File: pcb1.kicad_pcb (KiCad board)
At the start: 2 copper layers, 49.5 x 49.5 mm, 68 parts, among them P1 CONN_01X06, P10 M1, P11 M2, P12 CONN_01X02, P2 CONN_01X06, P3 CONN_01X06, P4 CONN_01X06, P5 UART, P6 SWD, Q1 IRF9540N, U1 74AHC1G14, U10 HL293D, U2 LTV-358T, U3 LTV-358T, U4 LM7812CT, U5 74AHC1G14, U6 STM32F030C6Tx, U7 LM7805CT, U8 LM1117-3.3, U9 HL293D

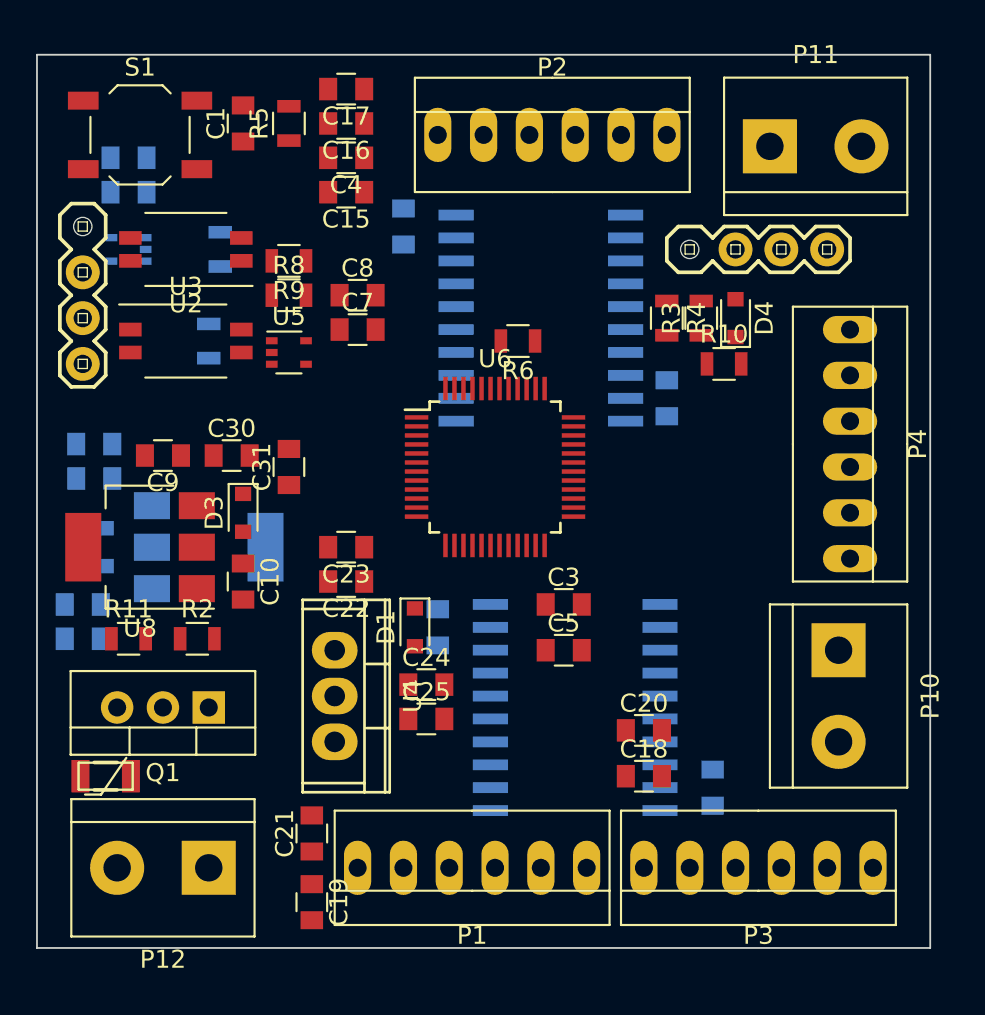
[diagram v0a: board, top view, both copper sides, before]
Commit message: 5x5
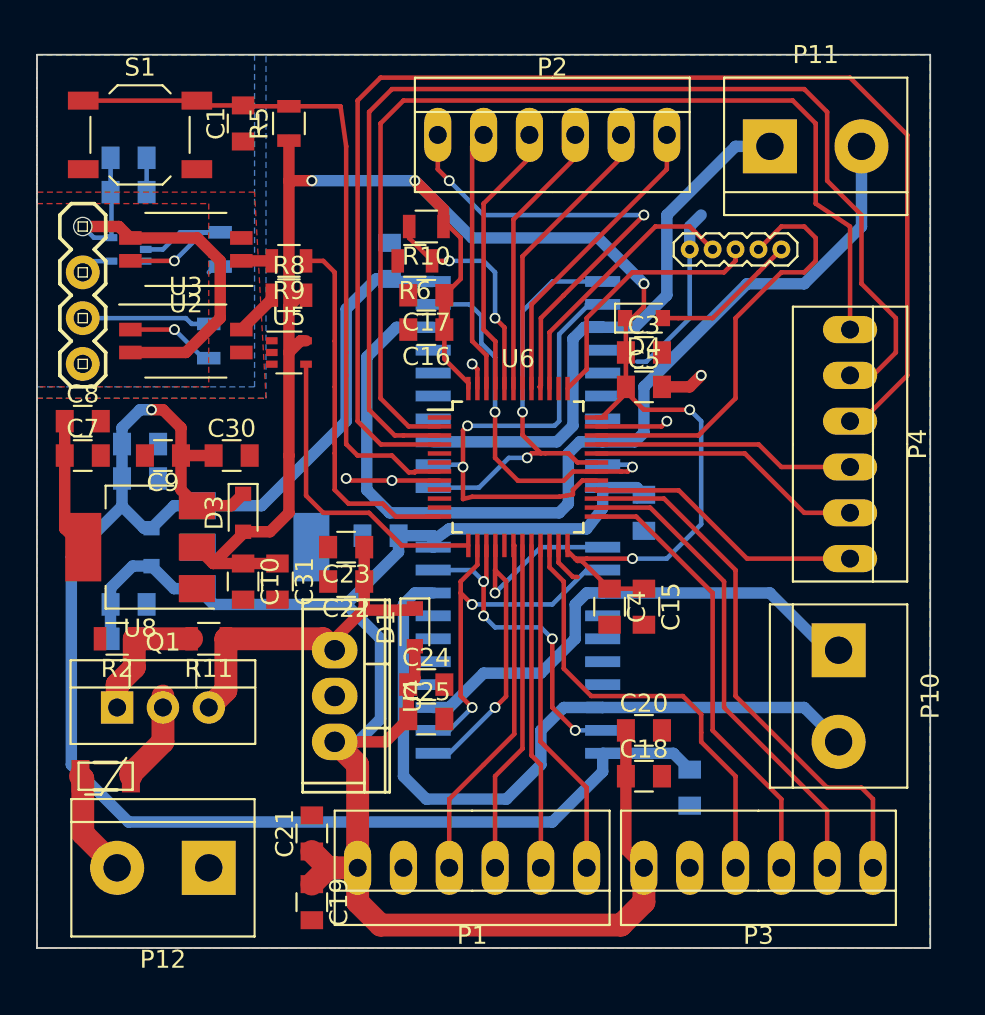
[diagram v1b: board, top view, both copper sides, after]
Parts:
- removed R3, R4: 100k, Resistors_SMD:R_0805
- P6: value SWD -> CONN_01X05; footprint SparkFun:SparkFun-1X04 -> SparkFun:SparkFun-1X05-1.27MM
- U6: value STM32F030C6Tx -> STM32F103C6Tx
- moved C4 28.9 mm to (219.7, 81.4), turned to 270 degrees
- moved C15 28.3 mm to (221.6, 81.4), turned to 270 degrees
- moved R10 18.2 mm to (209.6, 60.3), turned to 180 degrees
- moved C7 16.8 mm to (190.5, 73.0)
- moved C8 16.8 mm to (190.5, 71.1)
- moved C5 15.3 mm to (221.6, 69.2)
- moved C3 14.7 mm to (221.6, 67.3)
- moved C16 12.3 mm to (209.6, 66.0)
- moved C17 12.3 mm to (209.6, 64.1)
- moved R6 7.24 mm to (208.9, 62.2)
- moved C12 6.48 mm to (221.6, 76.2), turned to 270 degrees
- moved C31 6.38 mm to (201.3, 80.0), turned to 270 degrees
- moved C11 5.99 mm to (207.0, 77.5), turned to 180 degrees
- moved Q1 5.08 mm to (192.4, 87.0), turned to 0 degrees
- moved D4 5.08 mm to (221.6, 65.4), turned to 0 degrees
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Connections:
- P1 pad 1: Net-(P1-Pad1) -> /P11
- P2 pad 1: Net-(P2-Pad1) -> /P21
- P4 pad 5: Net-(P4-Pad5) -> /Enc4
- P6 pad 2: /SWCLK -> /SWO
- P6 pad 3: /SWDIO -> /SWCLK
- P6 pad 4: Net-(D4-Pad2) -> /SWDIO
- U6 pad 1: +3V3 -> (no net)
- U6 pad 17: Net-(U6-Pad17) -> (no net)
- U6 pad 2: Net-(U6-Pad2) -> /Enc0
- U6 pad 21: Net-(P3-Pad4) -> /P11
- U6 pad 22: Net-(P3-Pad3) -> Net-(P3-Pad4)
- U6 pad 25: Net-(P3-Pad2) -> Net-(P3-Pad3)
- U6 pad 26: Net-(P3-Pad1) -> Net-(P3-Pad2)
- U6 pad 27: Net-(P4-Pad6) -> Net-(P3-Pad1)
- U6 pad 28: Net-(P4-Pad5) -> Net-(P4-Pad6)
- U6 pad 3: Net-(U6-Pad3) -> /Enc1
- U6 pad 32: /Enc2 -> /Enc4
- U6 pad 35: Net-(U6-Pad35) -> GND
- U6 pad 36: Net-(U6-Pad36) -> +3V3
- U6 pad 38: Net-(U6-Pad38) -> (no net)
- U6 pad 39: Net-(P1-Pad1) -> /SWO
- U6 pad 4: Net-(U6-Pad4) -> /Enc2
- U6 pad 40: Net-(P2-Pad6) -> /P21
- U6 pad 41: Net-(P2-Pad5) -> Net-(P2-Pad6)
- U6 pad 42: Net-(P2-Pad4) -> Net-(P2-Pad5)
- U6 pad 43: Net-(P2-Pad3) -> Net-(P2-Pad4)
- U6 pad 45: Net-(P2-Pad2) -> Net-(P2-Pad3)
- U6 pad 46: Net-(P2-Pad1) -> Net-(P2-Pad2)
- U6 pad 5: Net-(U6-Pad5) -> (no net)
- U6 pad 6: Net-(U6-Pad6) -> (no net)
- U6 pad 9: Net-(U6-Pad9) -> (no net)
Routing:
- net +3V3: track 0.00 -> 109.8 mm, vias 0 -> 5
- net +12C: track 0.00 -> 98.9 mm
- net +5C: track 0.00 -> 98.9 mm, vias 0 -> 1
- net /Enc2: track 0.00 -> 72.7 mm
- net /Enc1: track 0.00 -> 65.4 mm
- net /Enc0: track 0.00 -> 56.8 mm
- net Net-(P11-Pad2): track 0.00 -> 53.8 mm
- net Net-(P10-Pad2): track 0.00 -> 41.0 mm
- net Net-(C1-Pad2): track 0.00 -> 39.0 mm
- net Net-(P11-Pad1): track 0.00 -> 33.6 mm
- net Net-(P3-Pad1): track 0.00 -> 30.1 mm
- net Net-(U10-Pad12): track 0.00 -> 27.8 mm, vias 0 -> 2
- net Net-(P10-Pad1): track 0.00 -> 27.5 mm
- net Net-(P3-Pad2): track 0.00 -> 27.0 mm
- net /P21: track 0.00 -> 26.4 mm, vias 0 -> 2
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- added copper zone on B.Cu, net GND
- added copper zone on F.Cu, net GND
- added copper zone on B.Cu, net VEE
- added copper zone on F.Cu, net VEE
